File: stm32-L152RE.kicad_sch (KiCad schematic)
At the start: 29 parts, among them J1 IDC 2x05 2.54mm, J2 JST SH, J3 TBD!!, J4 TDB, J5 TDB, SW1 SW_Push, U4 STM32L152RET6, U5 SIT1630AI-S4-DCC-32.768E, Y2 MAX7375AXR805

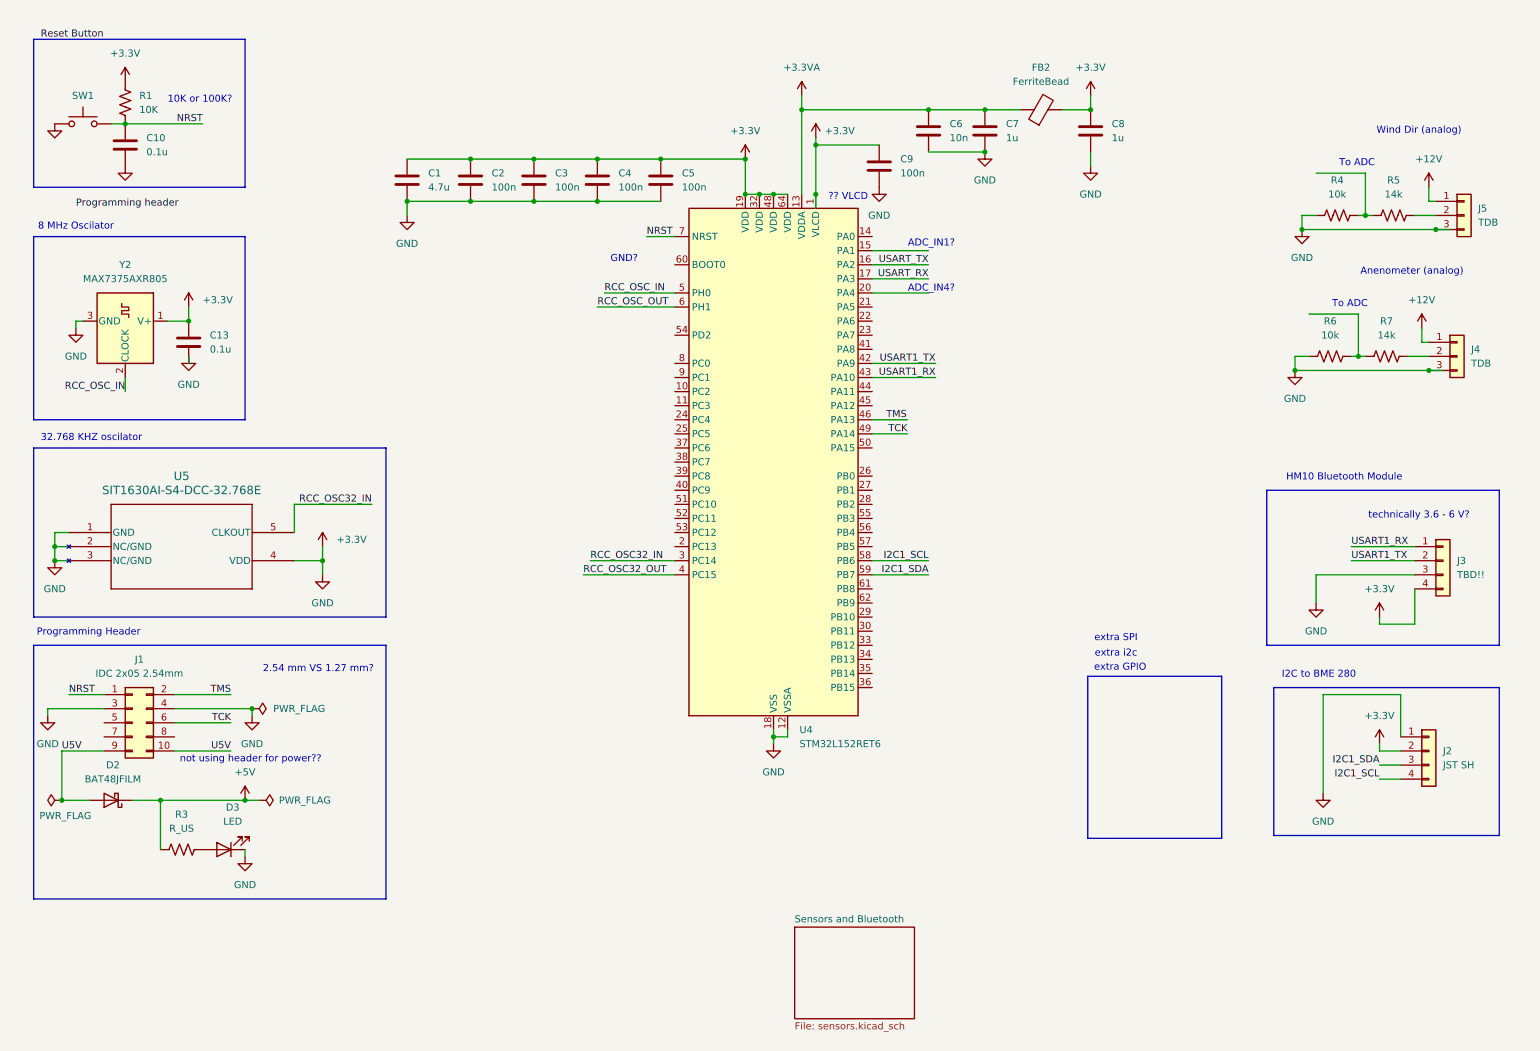
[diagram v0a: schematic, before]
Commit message: Add files via upload
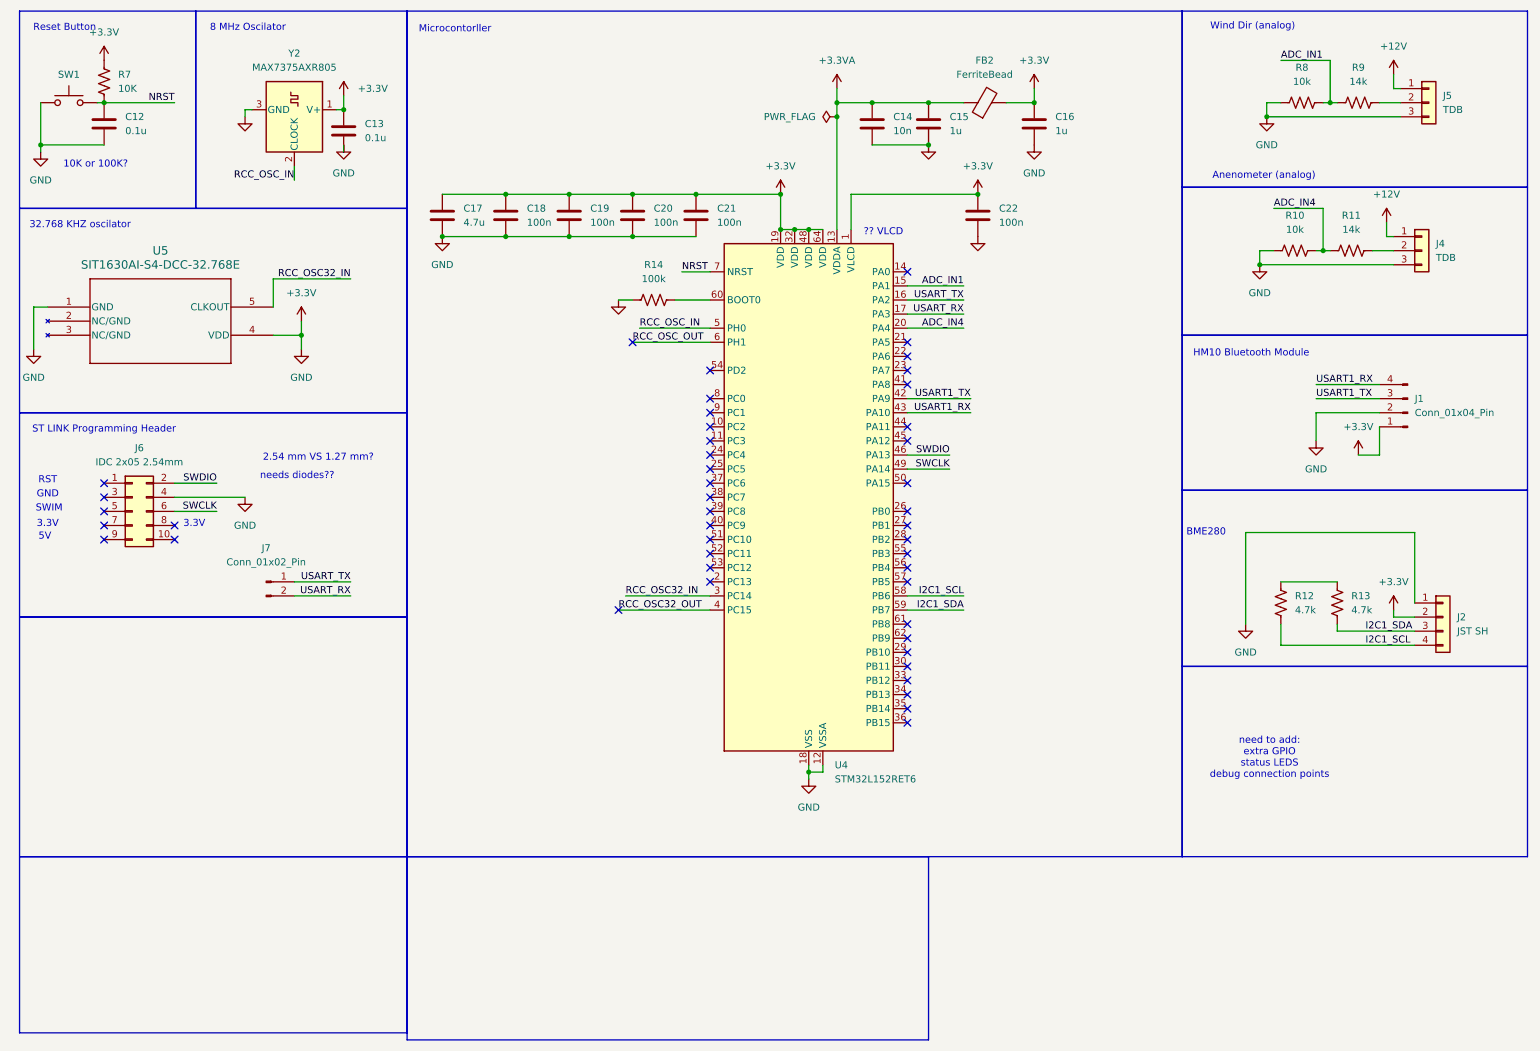
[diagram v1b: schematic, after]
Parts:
- removed D2: BAT48JFILM, Diode_SMD:D_SOD-323, symbol Diode:BAT48JFILM
- removed D3: LED, symbol Device:LED
- removed J1: IDC 2x05 2.54mm, Connector_IDC:IDC-Header_2x05_P2.54mm_Latch_Vertical, symbol Connector_Generic:Conn_02x05_Odd_Even
- removed J3: TBD!!, symbol Connector_Generic:Conn_01x04
- removed R3: R_US, symbol Device:R_US
- added J1: Conn_01x04_Pin, symbol Connector:Conn_01x04_Pin
- added J6: IDC 2x05 2.54mm, Connector_IDC:IDC-Header_2x05_P2.54mm_Latch_Vertical, symbol Connector_Generic:Conn_02x05_Odd_Even
- added J7: Conn_01x02_Pin, symbol Connector:Conn_01x02_Pin
- added R12, R13: 4.7k, symbol Device:R_US
- added R14: 100k, symbol Device:R_US
- renumbered C10 to C12, C6 to C14, C7 to C15, C8 to C16, C1 to C17, C2 to C18, C3 to C19, C4 to C20, C5 to C21, C9 to C22, R6 to R10, R7 to R11, R1 to R7, R4 to R8, R5 to R9
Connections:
- net +3.3V: now also J1.1 (Pin_1), J1.2 (Pin_2), J6.4 (Pin_4), R14.1; no longer U5.2 (NC/GND), U5.3 (NC/GND)
- net I2C1_SCL: now also R12.1
- net I2C1_SDA: now also R13.1
- net USART1_RX: now also J1.4 (Pin_4)
- net USART1_TX: now also J1.3 (Pin_3)
- net USART_RX: now also J7.2 (Pin_2)
- net USART_TX: now also J7.1 (Pin_1)
- net ADC_IN4: now reaches R10.2, R11.1
- net ADC_IN4: now also U4.20 (PA4)
- net ADC_IN1: now reaches R8.2, R9.1
- net ADC_IN1: now also U4.15 (PA1)
- net at U4.60 (BOOT0): now also R14.2
- net TCK renamed SWCLK
- net SWCLK: now also J6.6 (Pin_6)
- net TMS renamed SWDIO
- net SWDIO: now also J6.2 (Pin_2)
- new net: R12.2, R13.2
- no-connect marks 0 -> 46
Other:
- removed sheet Sensors and Bluetooth
- note added: "3.3V"
- note added: "5V"
- note added: "BME280"
- note added: "GND"
- note added: "Microcontorller"
- note added: "RST"
- note added: "Reset Button"
- note added: "ST LINK Programming Header"
- note added: "SWIM"
- note added: "need to add: extra GPIO status LEDS debug connection points"
- note added: "needs diodes??"
- note removed: "ADC_IN1?"
- note removed: "ADC_IN4?"
- note removed: "GND?"
- note removed: "I2C to BME 280"
- note removed: "Programming Header"
- note removed: "To ADC"
- note removed: "extra GPIO"
- note removed: "extra SPI"
- note removed: "extra i2c"
- note removed: "not using header for power??"
- note removed: "technically 3.6 - 6 V?"
- title: STM32L152RE, Programming Header etc  -> STM32L152RE Dev Board
- moved on the sheet: C12, C13, C14, C15, C16, C17, C18, C19, C20, C21, C22, FB2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

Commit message: updated schematic
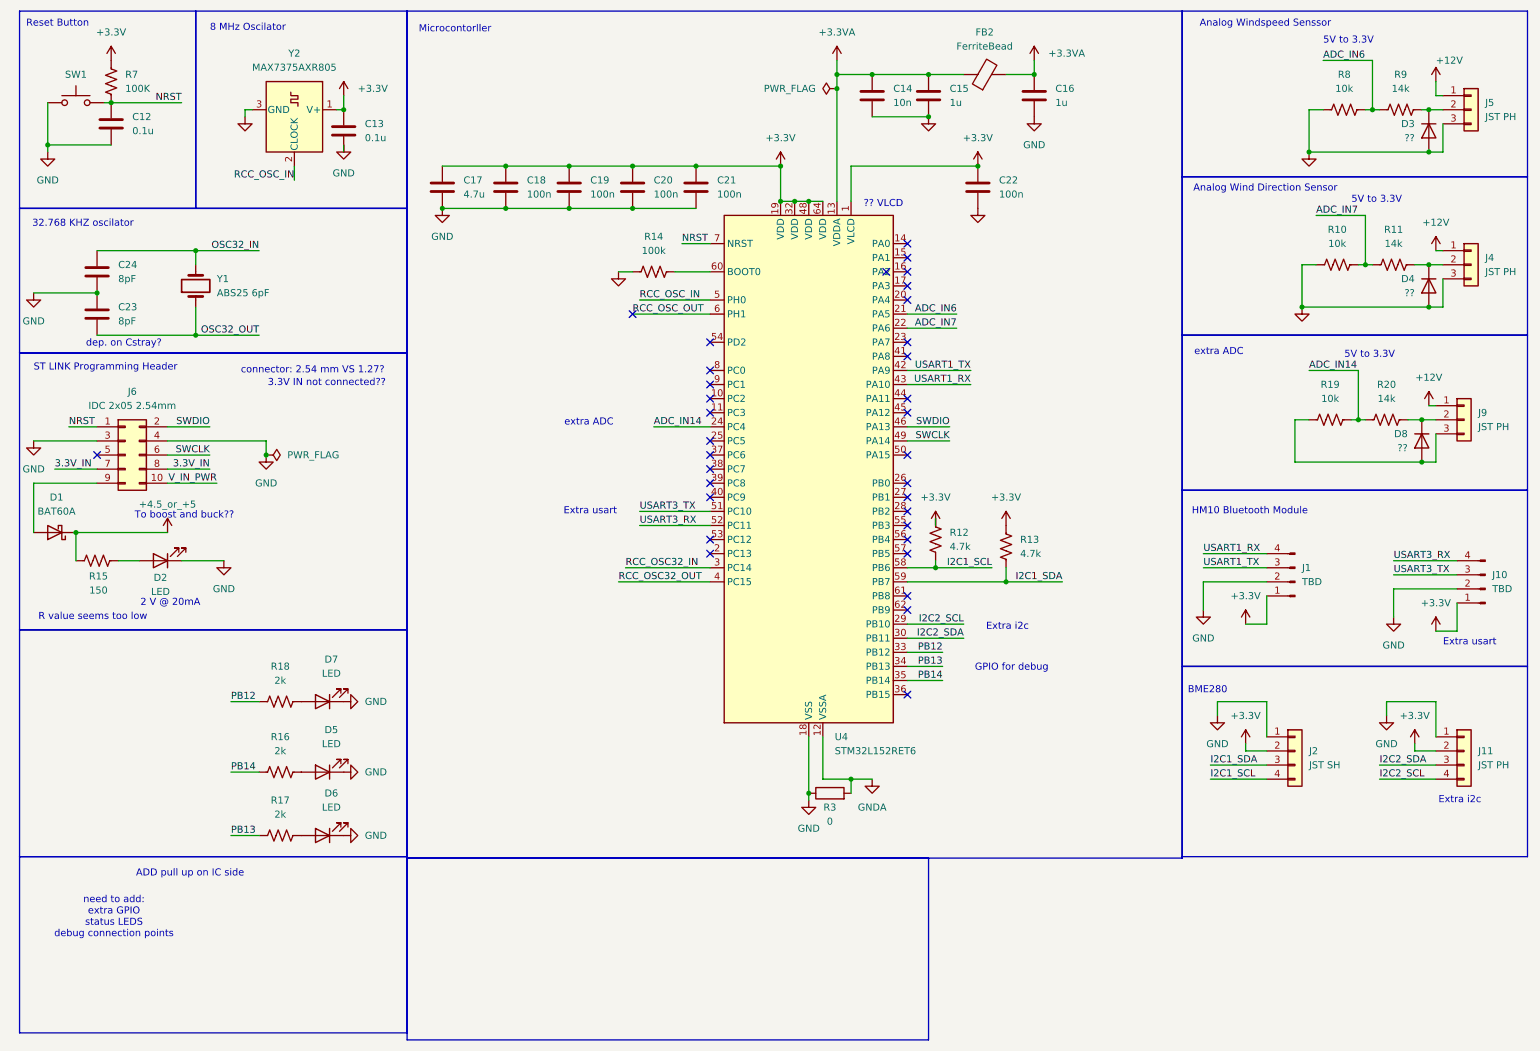
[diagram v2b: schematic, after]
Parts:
- removed J7: Conn_01x02_Pin, symbol Connector:Conn_01x02_Pin
- removed U5: SIT1630AI-S4-DCC-32.768E, FootprintLibrary:SOT_SiT1630-S_SIT, symbol SOT_SiT1630-S_SIT:SIT1630AI-S4-DCC-32.768E
- added C23, C24: 8pF, symbol Device:C
- added D1: BAT60A, Diode_SMD:D_SOD-323, symbol Diode:BAT60A
- added D2: LED, LED_SMD:LED_0805_2012Metric, symbol Device:LED
- added D3, D4, D8: ??, symbol Diode:1N4148WT
- added D5, D6, D7: LED, symbol Device:LED
- added J10: TBD, symbol Connector:Conn_01x04_Pin
- added J11: JST PH, Connector_JST:JST_PH_B2B-PH-K_1x02_P2.00mm_Vertical, symbol Connector_Generic:Conn_01x04
- added J9: JST PH, Connector_JST:JST_PH_B3B-PH-K_1x03_P2.00mm_Vertical, symbol Connector_Generic:Conn_01x03
- added R15: 150, symbol Device:R_US
- added R16, R17, R18: 2k, symbol Device:R_US
- added R19: 10k, symbol Device:R_US
- added R20: 14k, symbol Device:R_US
- added R3: 0, symbol Device:R
- added Y1: ABS25 6pF, Crystal:Crystal_SMD_Abracon_ABS25-4Pin_8.0x3.8mm, symbol Device:Crystal
- J1: value Conn_01x04_Pin -> TBD
- J4, J5: value TDB -> JST PH; footprint (none) -> Connector_JST:JST_PH_B3B-PH-K_1x03_P2.00mm_Vertical
- R7: value 10K -> 100K
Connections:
- net +12V: now also J9.1 (Pin_1)
- net +3.3V: now also R12.2, R13.2, J10.1 (Pin_1), J11.2 (Pin_2); no longer C12.2, C13.1, C14.2, C15.2, C16.1, C16.2, C17.2, C18.2, C19.2, C20.2, C21.2, C22.2, FB2.2, J1.2 (Pin_2), J2.1 (Pin_1), J4.3 (Pin_3), J5.3 (Pin_3), J6.4 (Pin_4), R10.1, R14.1, R8.1, SW1.1, U4.12 (VSSA), U4.18 (VSS), U4.31 (VSS), U4.47 (VSS), U4.63 (VSS), Y2.3 (GND)
- net +3.3VA: now also C16.1, FB2.2
- net NRST: now also J6.1 (Pin_1)
- net at J4.2 (Pin_2), R11.2: now also D4.1 (K)
- net at J5.2 (Pin_2), R9.2: now also D3.1 (K)
- net V_IN_PWR: now reaches J6.10 (Pin_10)
- net GND: now reaches J6.3 (Pin_3)
- net GND: now also C12.2, C13.1, C14.2, C15.2, C16.2, C17.2, C18.2, C19.2, C20.2, C21.2, C22.2, J1.2 (Pin_2), J2.1 (Pin_1), J4.3 (Pin_3), J5.3 (Pin_3), J6.4 (Pin_4), R10.1, R14.1, R8.1, SW1.1, U4.18 (VSS), U4.31 (VSS), U4.47 (VSS), U4.63 (VSS), Y2.3 (GND), C23.1, C24.2, D2.1 (K), D3.2 (A), D4.2 (A), D5.1 (K), D6.1 (K), D7.1 (K), J10.2 (Pin_2), J11.1 (Pin_1), R3.1
- net 3.3V_IN: now reaches J6.7 (Pin_7)
- net 3.3V_IN: now also J6.8 (Pin_8)
- net at J6.9 (Pin_9): now also D1.2 (A)
- net ADC_IN6: now reaches U4.21 (PA5)
- net ADC_IN6: now also R8.2, R9.1
- net ADC_IN7: now reaches U4.22 (PA6)
- net ADC_IN7: now also R10.2, R11.1
- net ADC_IN14: now reaches U4.24 (PC4)
- net ADC_IN14: now also R19.2, R20.1
- net I2C2_SCL: now reaches U4.29 (PB10)
- net I2C2_SCL: now also J11.4 (Pin_4)
- net I2C2_SDA: now reaches U4.30 (PB11)
- net I2C2_SDA: now also J11.3 (Pin_3)
- net PB12: now reaches U4.33 (PB12)
- net PB12: now also R18.1
- net PB13: now reaches U4.34 (PB13)
- net PB13: now also R17.1
- net PB14: now reaches U4.35 (PB14)
- net PB14: now also R16.1
- net USART3_TX: now reaches U4.51 (PC10)
- net USART3_TX: now also J10.3 (Pin_3)
- net USART3_RX: now reaches U4.52 (PC11)
- net USART3_RX: now also J10.4 (Pin_4)
- removed net ADC_IN1: R8.2, R9.1, U4.15 (PA1)
- removed net ADC_IN4: R10.2, R11.1, U4.20 (PA4)
- net USART_RX: no longer names the net of U4.17 (PA3)
- net USART_TX: no longer names the net of U4.16 (PA2)
- new net: D8.2 (A), J9.3 (Pin_3), R19.1
- new net: D6.2 (A), R17.2
- new net: D8.1 (K), J9.2 (Pin_2), R20.2
- new net: D7.2 (A), R18.2
- new net: D2.2 (A), R15.1
- new net: D5.2 (A), R16.2
- new net +4.5_or_+5: D1.1 (K), R15.2
- new net GNDA: R3.2, U4.12 (VSSA)
- new net OSC32_IN: C24.1, Y1.2
- new net OSC32_OUT: C23.2, Y1.1
- no-connect marks 46 -> 34
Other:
- note added: "2 V @ 20mA"
- note added: "3.3V IN not connected??"
- note added: "5V to 3.3V"
- note added: "ADD pull up on IC side"
- note added: "Analog Wind Direction Sensor"
- note added: "Analog Windspeed Senssor"
- note added: "Extra i2c"
- note added: "Extra usart"
- note added: "GPIO for debug"
- note added: "R value seems too low"
- note added: "To boost and buck??"
- note added: "connector: 2.54 mm VS 1.27?"
- note added: "dep. on Cstray?"
- note added: "extra ADC"
- note removed: "10K or 100K?"
- note removed: "2.54 mm VS 1.27 mm?"
- note removed: "3.3V"
- note removed: "5V"
- note removed: "Anenometer (analog)"
- note removed: "GND"
- note removed: "RST"
- note removed: "SWIM"
- note removed: "Wind Dir (analog)"
- note removed: "needs diodes??"
- moved on the sheet: C12, C14, C15, C16, C17, C18, C19, C20, C21, C22, FB2, J1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
